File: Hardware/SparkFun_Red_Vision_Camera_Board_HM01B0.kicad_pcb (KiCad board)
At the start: 4 copper layers, 22.9 x 35.6 mm, 115 parts, among them J1 Conn_01x09, J2 Conn_01x09, J3 Conn_01x09, J4 HM01B0, Q1 RE1C002UNTCL, Q2 RE1C002UNTCL, Q3 RE1C002UNTCL, Q4 RE1C002UNTCL, U1 HM01B0, U2 RT9080-2.8V, Y1 24MHz

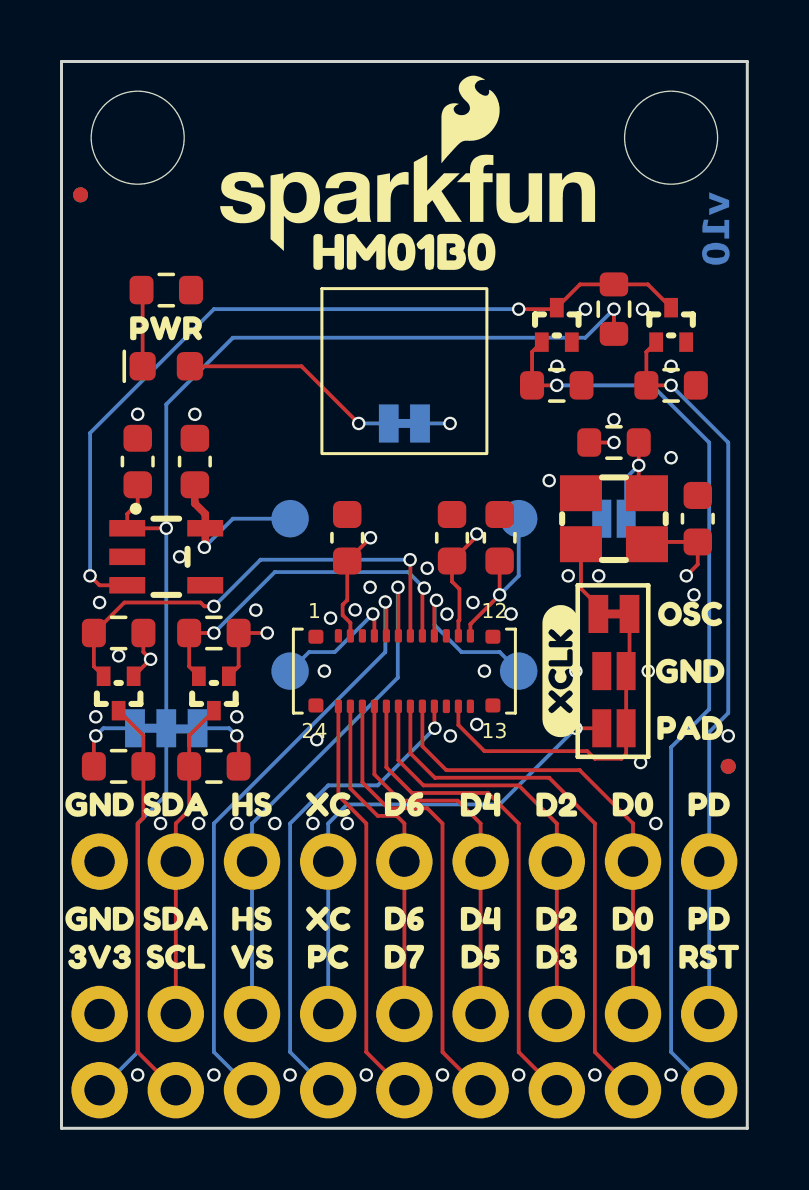
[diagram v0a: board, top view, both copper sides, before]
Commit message: Update libraries
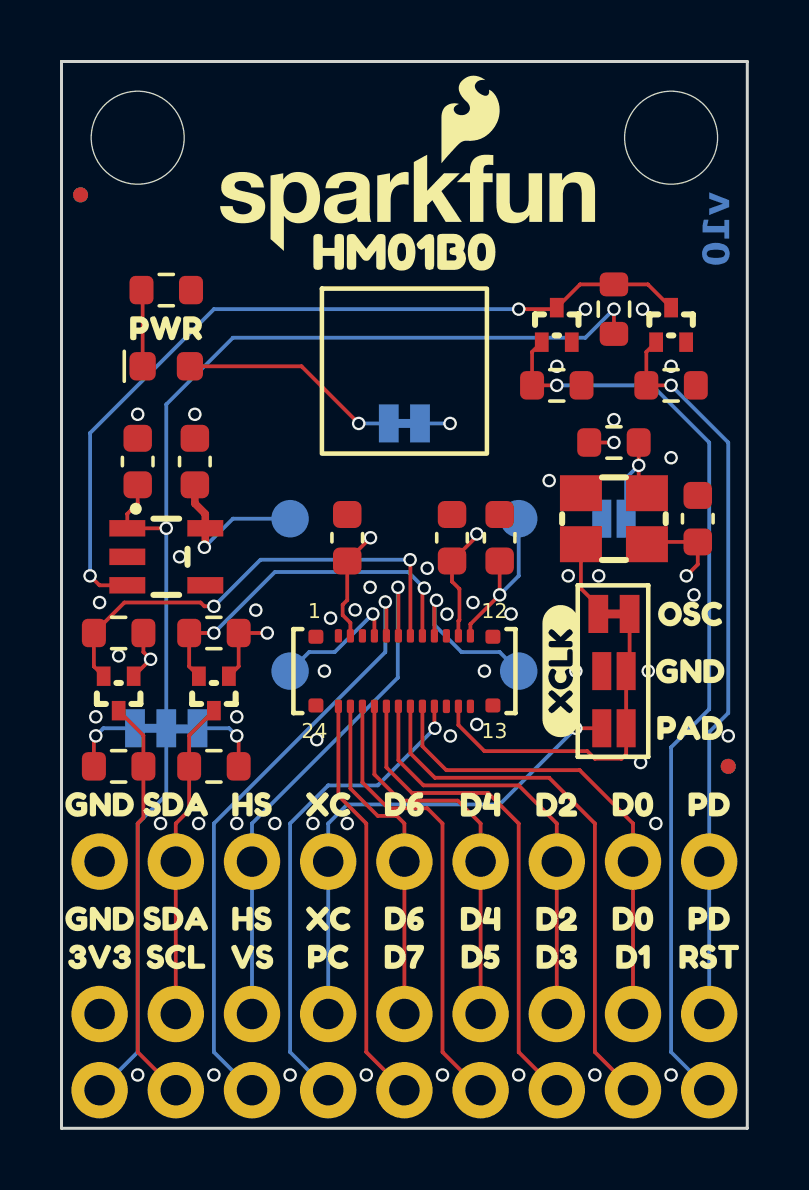
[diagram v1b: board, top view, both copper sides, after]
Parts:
- J4: footprint lcd-tft:Socket_2x12_0.4mm-pitch_5055502420 -> SparkFun-Connector:FPC_2x12-1MP_P0.4mm
- U1: footprint lcd-tft:HM01B0-ANA-00FT870 -> SparkFun-Camera:HM01B0-ANA-00FT870
